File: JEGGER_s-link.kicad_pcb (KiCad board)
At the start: 2 copper layers, 37.6 x 16.1 mm, 43 parts, among them J1 USB, J2 TC, J3 PINH, J4 RX, J5 TX, P1 STM, Q1 S9013, U1 USBLC6-4, U2 MCP1700T-3302E/TT, U3 STM32F103CBTx, Y1 8Mhz

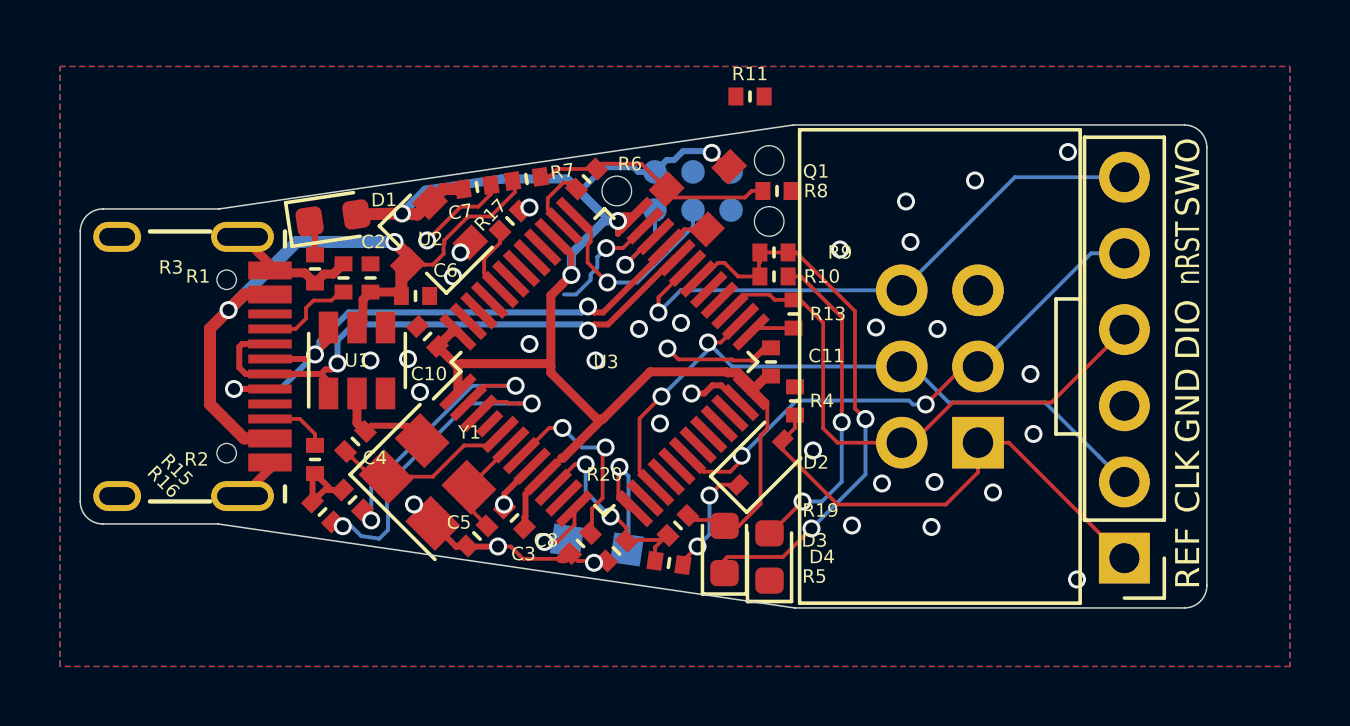
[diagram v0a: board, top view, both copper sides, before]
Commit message: push
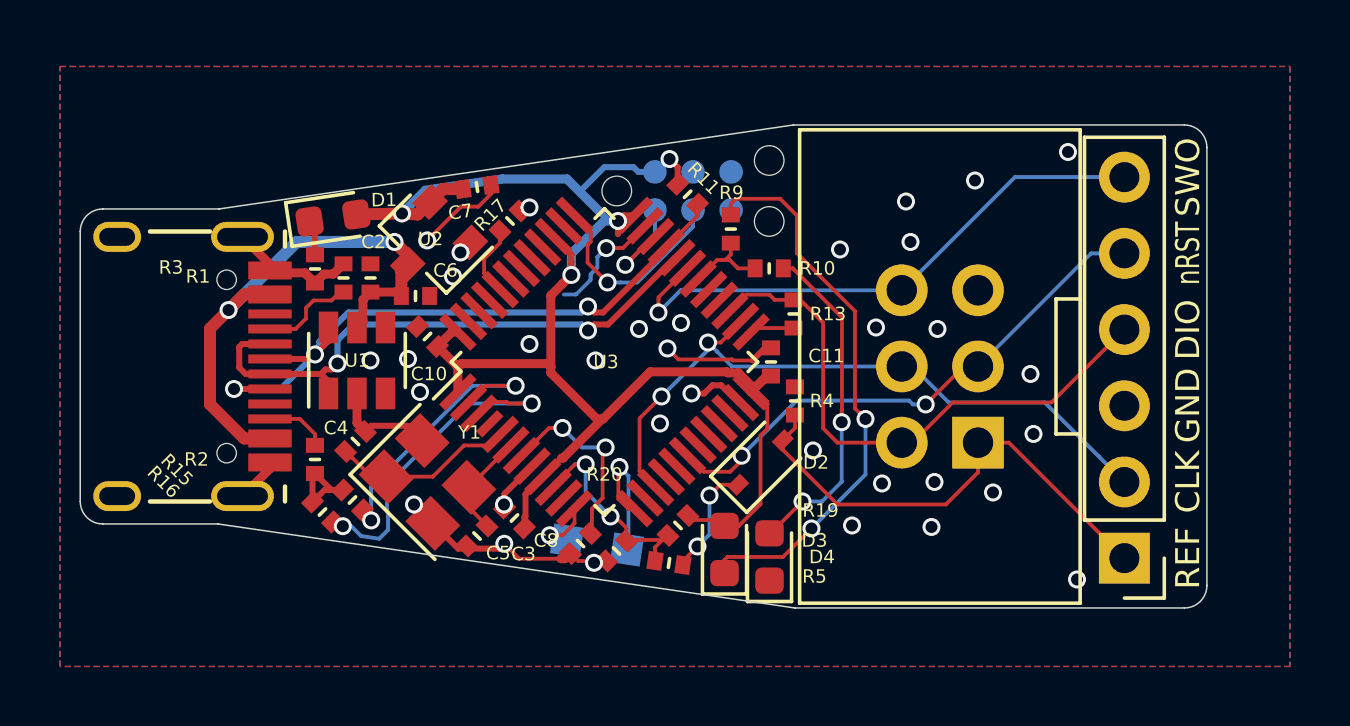
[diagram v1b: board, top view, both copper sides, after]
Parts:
- removed Q1: S9013, Package_TO_SOT_SMD:SOT-23
- removed R6: 100, otter:R_0402
- removed R7: 10k, otter:R_0402
- removed R8: 36k, otter:R_0402
- moved R11 3.87 mm to (120.9, 94.3), turned to 315 degrees
- moved R9 1.64 mm to (122.4, 95.4), turned to 90 degrees
- moved R10 0.31 mm to (123.6, 96.7)
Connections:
- R11 pad 1: Net-(Q1-Pad2) -> +3V3
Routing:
- net Net-(Q1-Pad1): track 8.15 -> 0.00 mm
- net VBUS: track 23.7 -> 18.5 mm
- net Net-(D3-Pad1): track 15.7 -> 18.9 mm
- net USB_RENUM: track 2.41 -> 0.00 mm
- net +3V3: track 54.3 -> 52.9 mm
